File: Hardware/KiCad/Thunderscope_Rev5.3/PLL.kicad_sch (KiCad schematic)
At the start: 47 parts, among them J6 UFL, J7 UFL, U7 ZL30260LDG1, Y1 10MHz

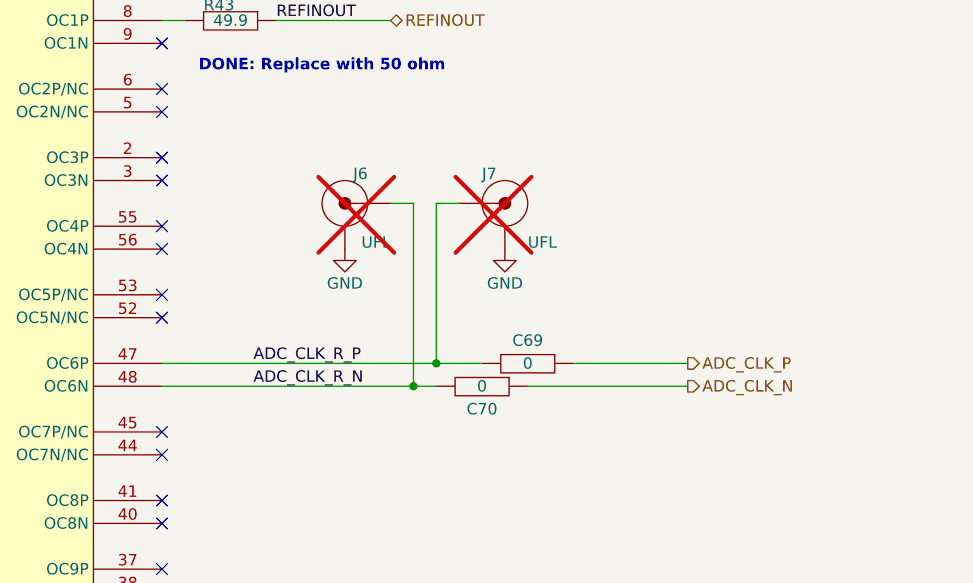
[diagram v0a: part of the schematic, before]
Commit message: Removed Clock Test Ports, Closing #406
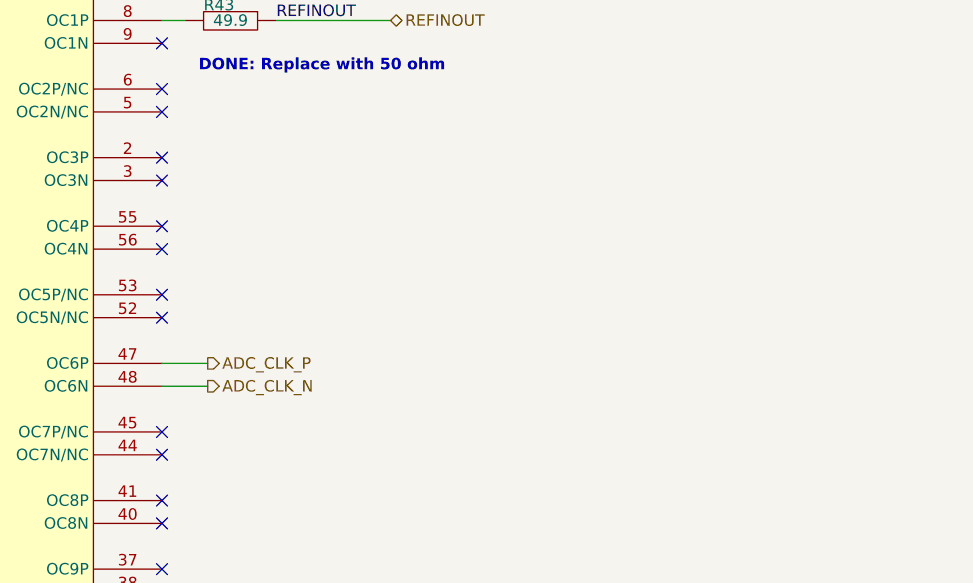
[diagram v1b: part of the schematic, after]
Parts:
- removed C69, C70: 0, Thunderscope_Rev5:GEN_R_0402, symbol Thunderscope_Rev5:RES 0 OHM 1/16W 0402
- removed J6, J7: UFL, Thunderscope_Rev5:TE_2334884-1, symbol Thunderscope_Rev5:UFL Jack SMD
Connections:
- net ADC_CLK_R_N is gone; now on net ADC_CLK_N: U7.48 (OC6N)
- net ADC_CLK_R_P is gone; now on net ADC_CLK_P: U7.47 (OC6P)
